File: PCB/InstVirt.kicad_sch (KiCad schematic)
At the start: 45 parts, among them J1 Conn_01x20_Pin, J2 Conn_01x20_Pin, J3 Conn_01x08_Socket, J4 Conn_01x08_Socket, Q1 BC548, Q2 BC548, Q3 BC548, Q4 BC548, Q5 BC548, Q6 BC548, Q7 BC548, Q8 BC548, U1 4051

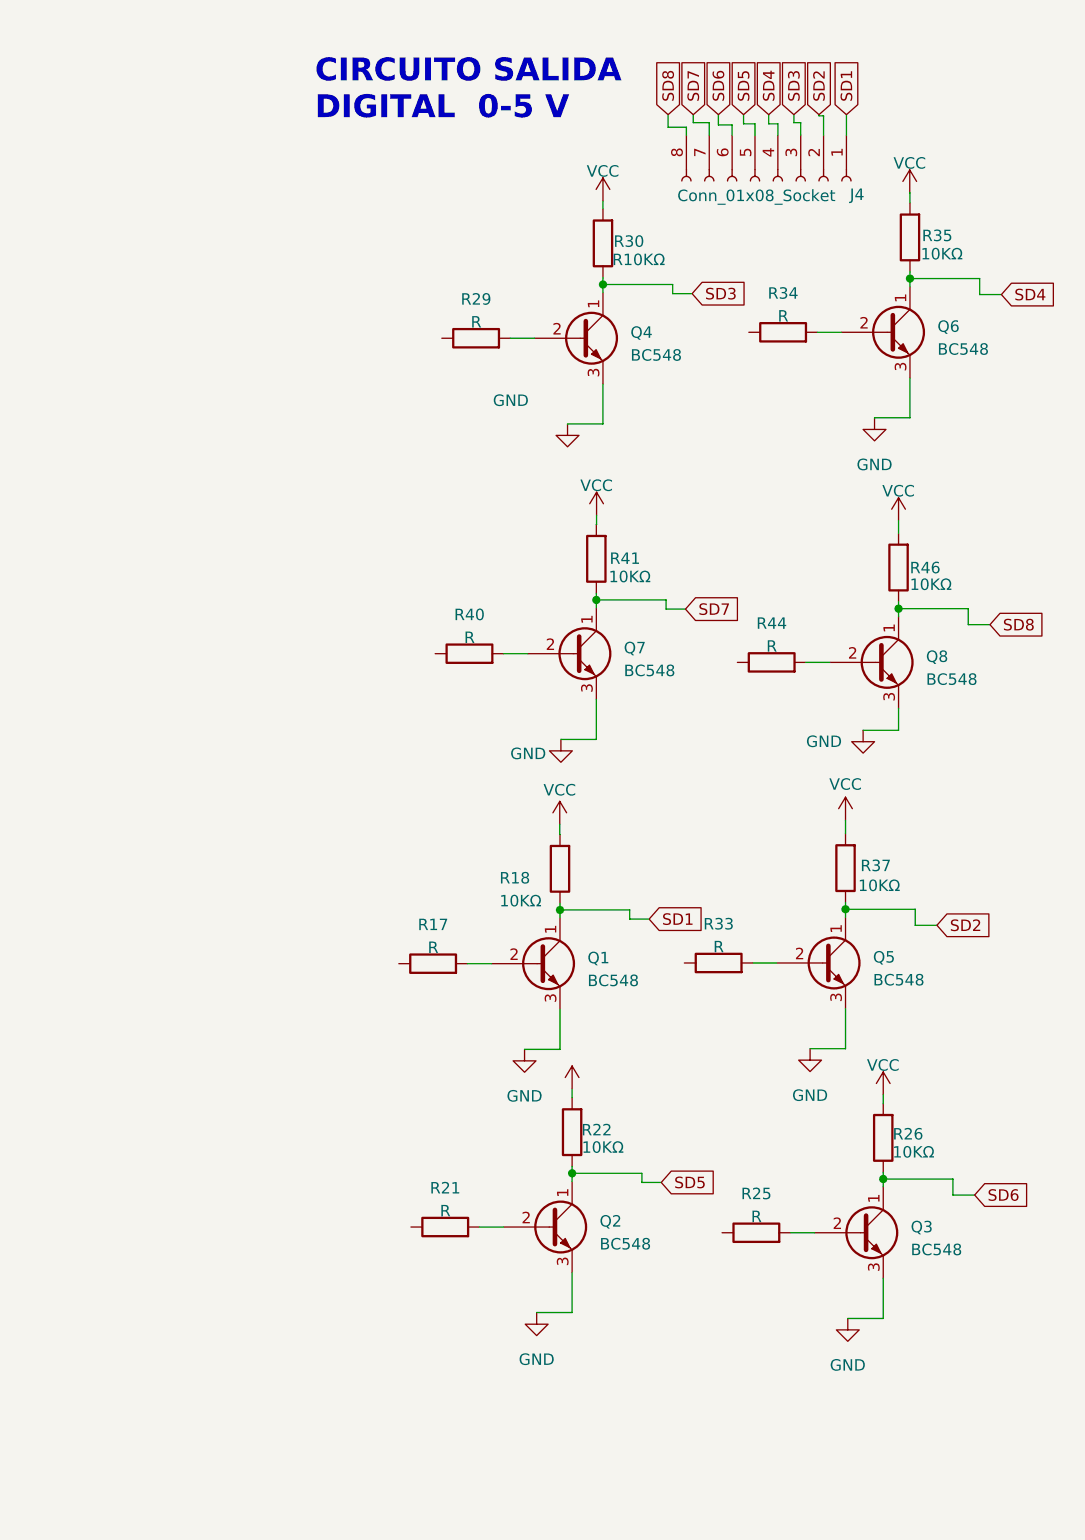
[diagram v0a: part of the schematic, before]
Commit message: Actualizo circuito PCB
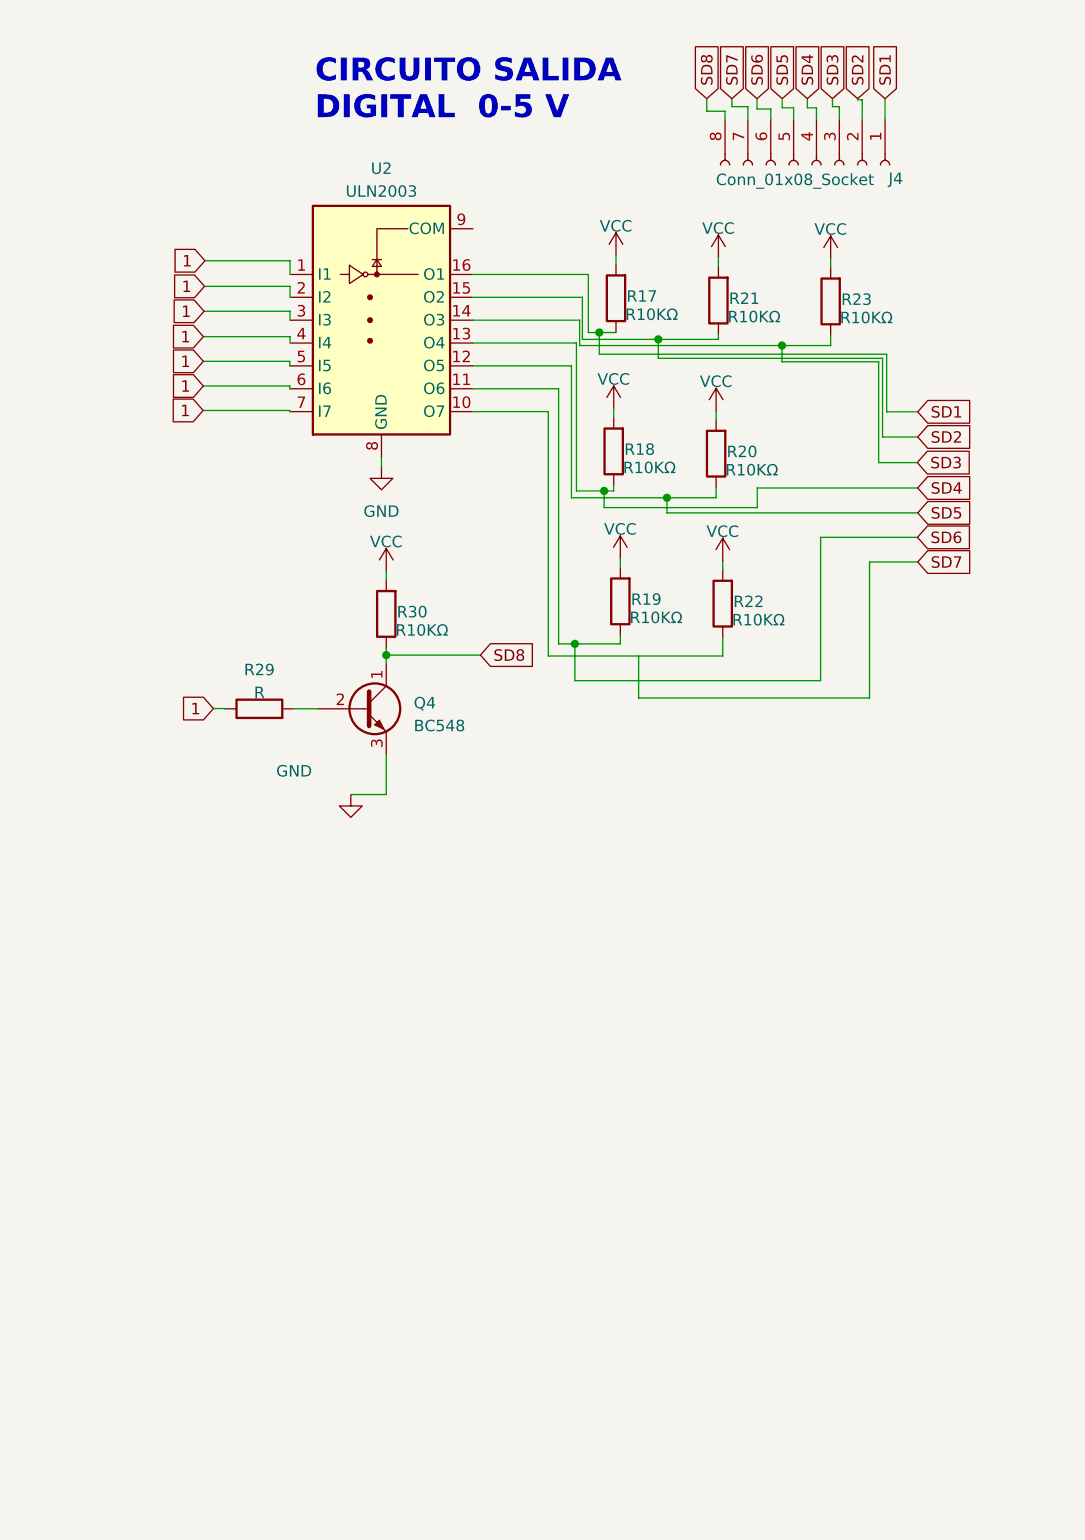
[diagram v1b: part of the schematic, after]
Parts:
- removed Q1, Q2, Q3, Q5, Q6, Q7, Q8: BC548, Package_TO_SOT_THT:TO-92_Inline, symbol Transistor_BJT:BC548
- removed R25, R33, R34, R40, R44: R, symbol Device:R
- removed R26, R35, R37, R41, R46: 10KΩ, symbol Device:R
- added R19, R20, R23: R10KΩ, symbol Device:R
- added U2: ULN2003, symbol Transistor_Array:ULN2003
- R17, R21: value R -> R10KΩ
- R18, R22: value 10KΩ -> R10KΩ
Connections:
- net GND: now also U2.8 (GND)
- net SD1: now also R17.1, U2.16 (O1); no longer R18.1
- net SD2: now also R21.1, U2.15 (O2)
- net SD3: now also R23.1, U2.14 (O3); no longer Q4.1 (C), R30.1
- net SD4: now also R18.1, U2.13 (O4)
- net SD5: now also R20.1, U2.12 (O5); no longer R22.1
- net SD6: now also R19.1, U2.11 (O6)
- net SD8: now also Q4.1 (C), R30.1
- net VCC: now also R17.2, R21.2, R19.2, R20.2, R23.2
- net 1: now reaches R29.1
- net 1: now also U2.1 (I1), U2.2 (I2), U2.3 (I3), U2.4 (I4), U2.5 (I5), U2.6 (I6), U2.7 (I7)
- new net: R22.1, U2.10 (O7)
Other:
- moved on the sheet: J4, Q4, R29, R30
